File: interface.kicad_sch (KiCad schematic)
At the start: 59 parts, among them J5 5034801200, SW1 TS35CA, U10 LIS2DW12TR, U11 AP3602AKTR-G1, U8 DRV2603RUNT, U9 TPS61040DBV

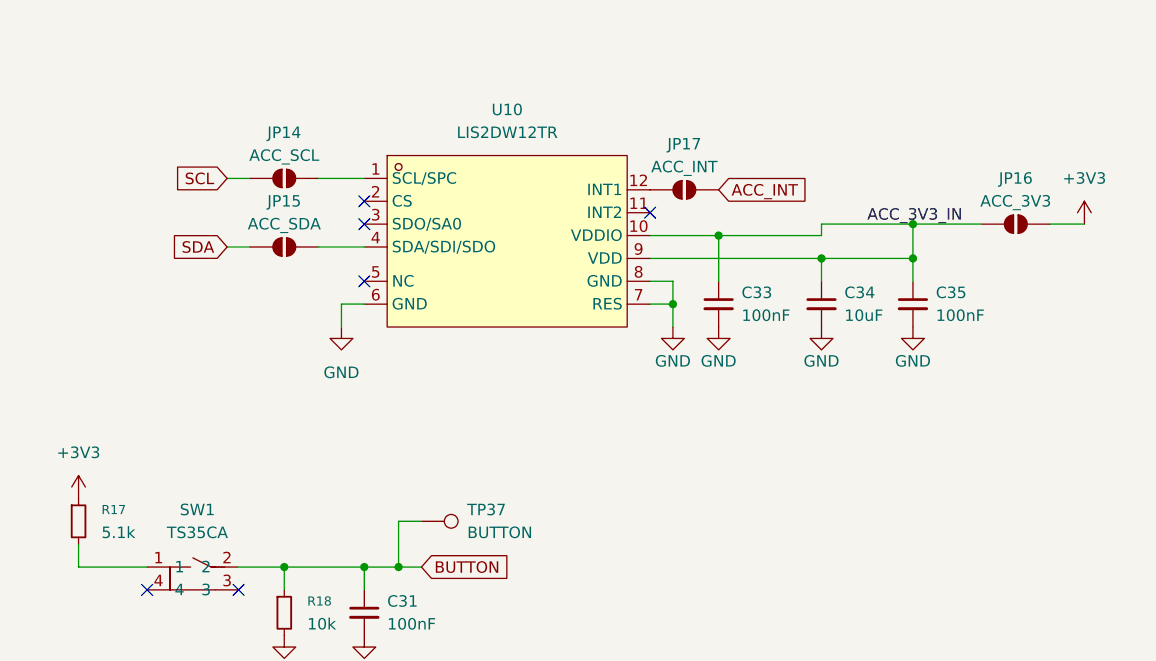
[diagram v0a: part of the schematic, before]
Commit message: fixups before manufacturing pt1
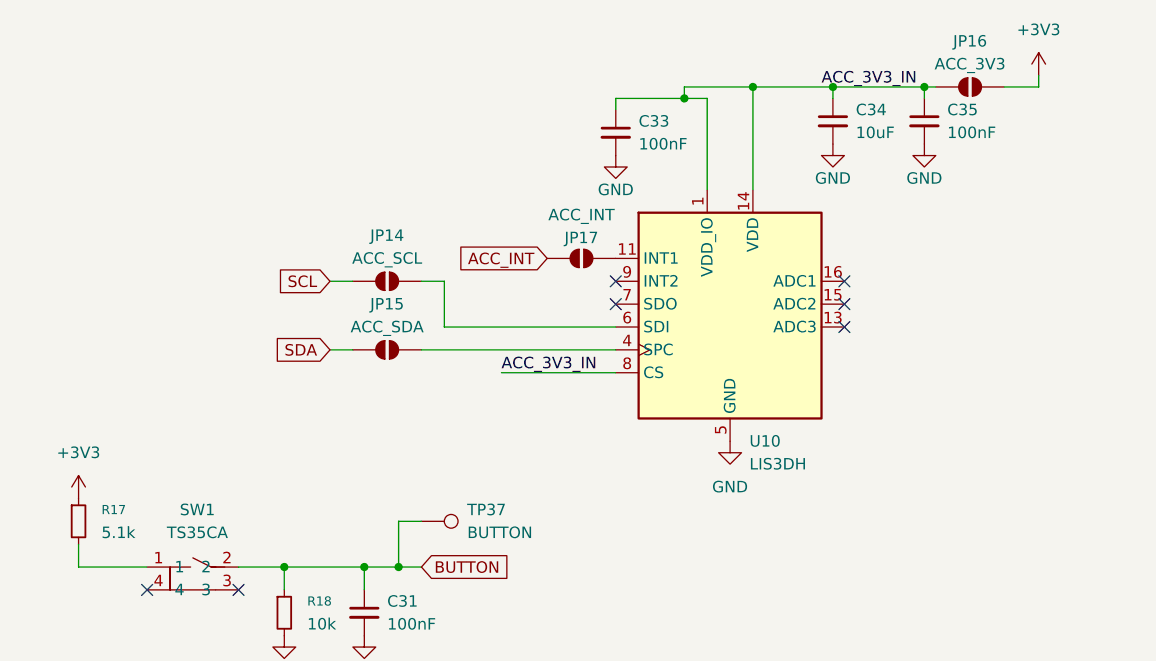
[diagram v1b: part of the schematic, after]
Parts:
- removed U10: LIS2DW12TR, LIS2DW12TR:LGA-12_L2.0-W2.0-P0.50-BL, symbol LIS2DW12TR:LIS2DW12TR
- added U10: LIS3DH, Package_LGA:LGA-16_3x3mm_P0.5mm_LayoutBorder3x5y, symbol Sensor_Motion:LIS3DH
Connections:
- net ACC_3V3_IN: now also U10.1 (VDD_IO), U10.14 (VDD), U10.8 (CS)
- net GND: now also U10.10 (GND), U10.12 (GND), U10.5 (GND)
- net at JP17.1 (A): now also U10.11 (INT1)
- net at JP15.2 (B): now also U10.4 (SPC)
- net at JP14.2 (B): now also U10.6 (SDI)
- no-connect marks 8 -> 9
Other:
- moved on the sheet: C33, C34, C35, JP14, JP15, JP16, JP17
